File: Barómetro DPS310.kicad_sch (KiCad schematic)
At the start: 6 parts, among them U5 DPS310XTSA1

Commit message: Cantidad de errores en la PCB: 29
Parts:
- C24, C25: footprint easyeda2kicad:C0402 -> ARLISS-footprints:C0402
- U5: footprint easyeda2kicad:LGA-8_DPS310XTSA1 -> ARLISS-footprints:LGA-8_DPS310XTSA1
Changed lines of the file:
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@@
 			)
 		)
-		(property "Footprint" "easyeda2kicad:C0402"
+		(property "Footprint" "ARLISS-footprints:C0402"
 			(at 210.82 100.33 0)
 			(hide yes)
@@
 			)
 		)
-		(property "Footprint" "easyeda2kicad:LGA-8_DPS310XTSA1"
+		(property "Footprint" "ARLISS-footprints:LGA-8_DPS310XTSA1"
 			(at 166.37 105.41 0)
 			(hide yes)
@@
 			)
 		)
-		(property "Footprint" "easyeda2kicad:C0402"
+		(property "Footprint" "ARLISS-footprints:C0402"
 			(at 191.77 81.28 0)
 			(hide yes)

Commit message: Cantidad de errores de la placa: 05
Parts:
- R4, R5: footprint easyeda2kicad:R0603 -> ARLISS-footprints:R0603
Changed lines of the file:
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@@
 			)
 		)
-		(property "Footprint" "easyeda2kicad:R0603"
+		(property "Footprint" "ARLISS-footprints:R0603"
 			(at 142.24 88.9 0)
 			(hide yes)
@@
 			)
 		)
-		(property "Footprint" "easyeda2kicad:R0603"
+		(property "Footprint" "ARLISS-footprints:R0603"
 			(at 151.13 87.63 0)
 			(hide yes)

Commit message: Cantidad de errores en la placa: 04
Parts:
- R1: footprint (none) -> ARLISS-footprints:R0603; LCSC Part (none) -> C5552302
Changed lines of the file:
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@@
 			)
 		)
-		(property "Footprint" ""
+		(property "Footprint" "ARLISS-footprints:R0603"
 			(at 179.832 105.41 90)
 			(hide yes)
@@
 			)
 		)
-		(property "Datasheet" ""
+		(property "Datasheet" "https://www.lcsc.com/datasheet/C5552302.pdf?spm=wm.sxq.pdf.fd___wm.fly.bg.1.cbh&lcsc_vid=FVBZXlJVElFWAVdTTgAPVAcHR1hXAlIFT1cMUAFWQVYxVlNeRlVfVFdeR1NaXzsOAxUeFF5JWBYZEEoKFBINSQcJGk4dAgUUFAk%3D"
 			(at 181.61 105.41 0)
 			(hide yes)
@@
 			(at 181.61 105.41 0)
 			(hide yes)
+			(show_name no)
+			(do_not_autoplace no)
+			(effects
+				(font
+					(size 1.27 1.27)
+				)
+			)
+		)
+		(property "LCSC Part" "C5552302"
+			(at 181.61 105.41 0)
+			(hide yes)

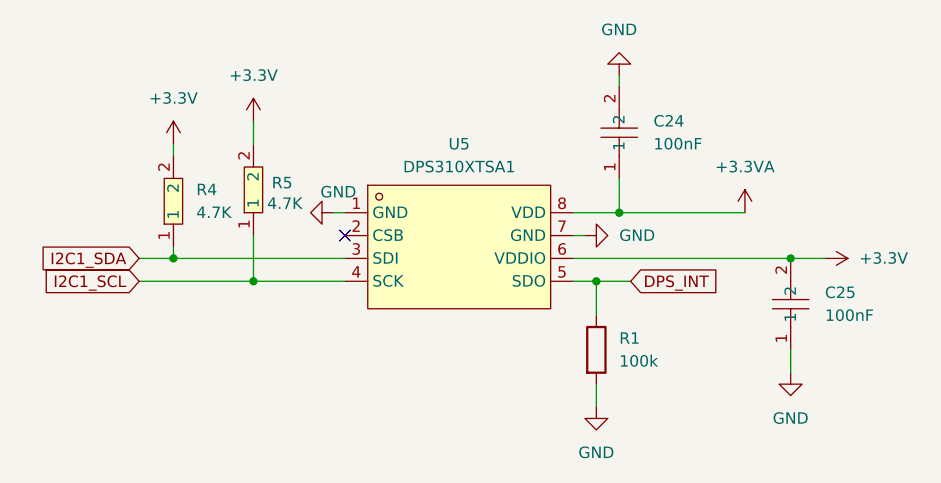
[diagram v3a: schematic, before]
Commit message: PCB ordenada V1
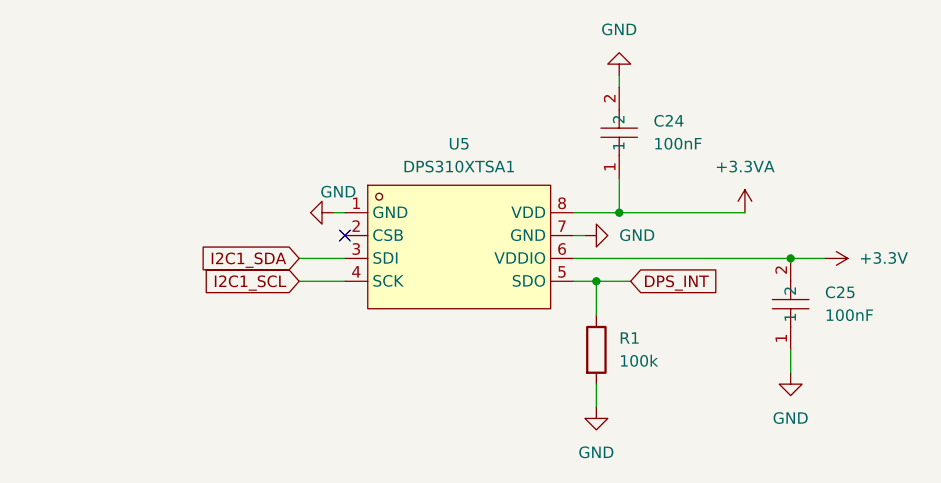
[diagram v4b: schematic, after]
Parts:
- removed R4, R5: 4.7K, ARLISS-footprints:R0603, symbol CANSAT_STM32_symbols:RC0603FR-074K7L

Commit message: Primer Ruteo de PCB
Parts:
- C24, C25: footprint ARLISS-footprints:C0402 -> Capacitor_SMD:C_0402_1005Metric_Pad0.74x0.62mm_HandSolder
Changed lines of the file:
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@@
 			)
 		)
-		(property "Footprint" "ARLISS-footprints:C0402"
+		(property "Footprint" "Capacitor_SMD:C_0402_1005Metric_Pad0.74x0.62mm_HandSolder"
 			(at 210.82 100.33 0)
 			(hide yes)
@@
 			)
 		)
-		(property "Footprint" "ARLISS-footprints:C0402"
+		(property "Footprint" "Capacitor_SMD:C_0402_1005Metric_Pad0.74x0.62mm_HandSolder"
 			(at 191.77 81.28 0)
 			(hide yes)

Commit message: Arreglos de esquemático
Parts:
- R1: footprint ARLISS-footprints:R0603 -> Resistor_SMD:R_0603_1608Metric_Pad0.98x0.95mm_HandSolder
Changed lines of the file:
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@@
 			)
 		)
-		(property "Footprint" "ARLISS-footprints:R0603"
+		(property "Footprint" "Resistor_SMD:R_0603_1608Metric_Pad0.98x0.95mm_HandSolder"
 			(at 179.832 105.41 90)
 			(hide yes)
